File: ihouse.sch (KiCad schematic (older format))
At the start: 7 parts

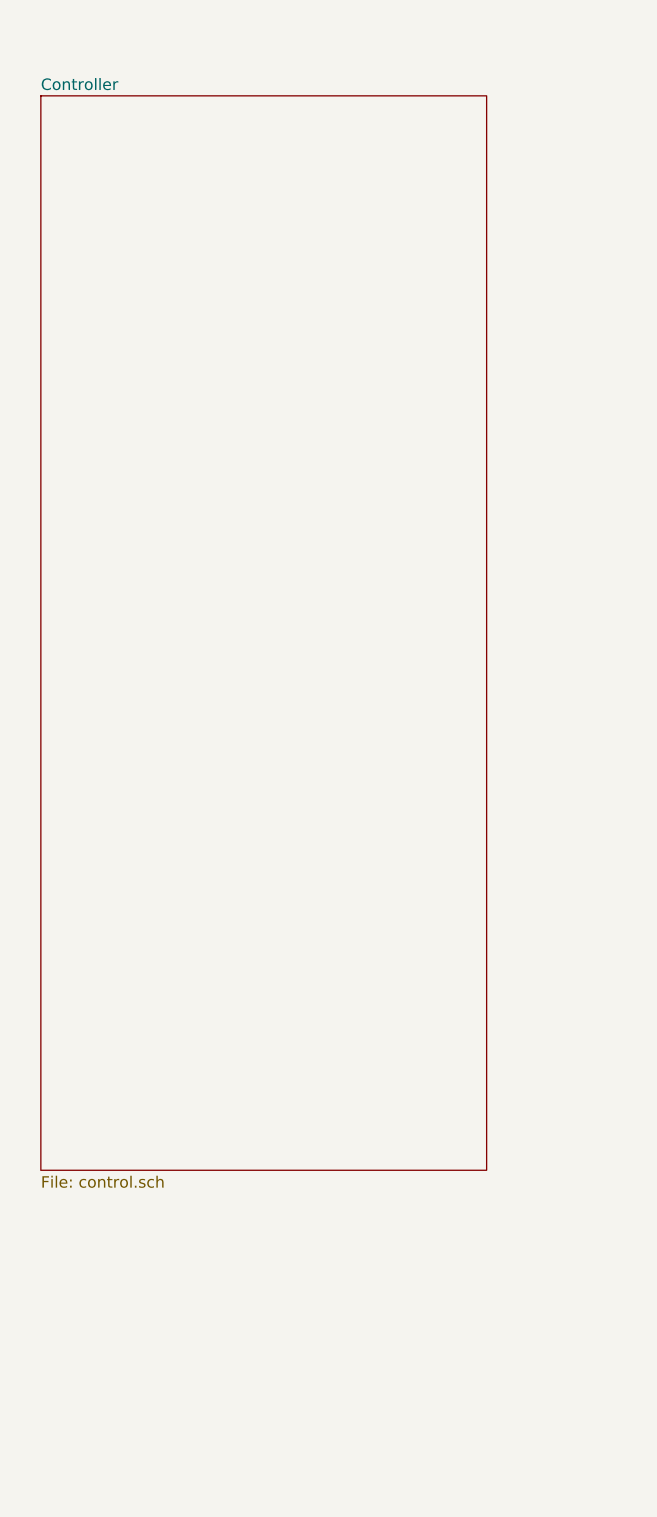
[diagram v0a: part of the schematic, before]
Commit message: tarpinis kommitas
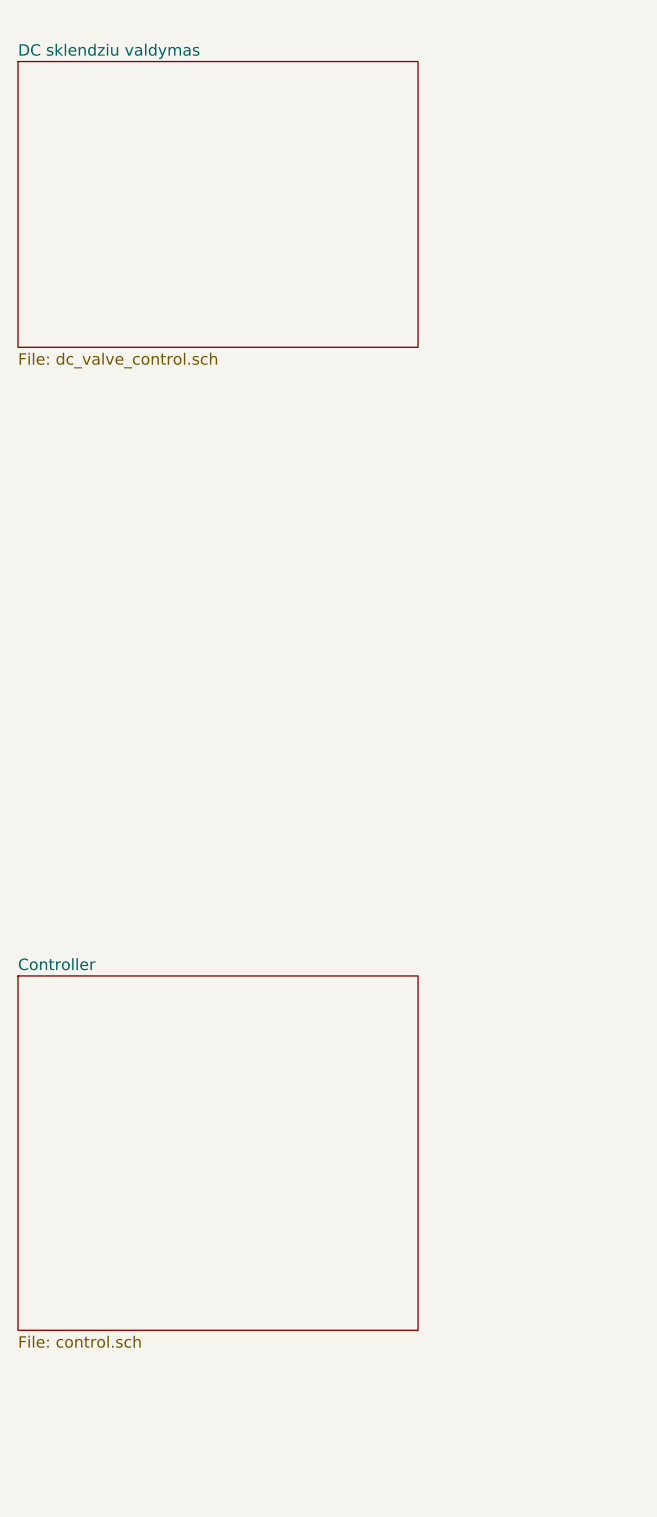
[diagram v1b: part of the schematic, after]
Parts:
- gave numbers to parts that had none: 7
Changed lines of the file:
@@
 $Descr A4 11693 8268
 encoding utf-8
-Sheet 1 3
+Sheet 1 4
 Title ""
 Date ""
@@
 $EndDescr
 $Sheet
-S 2100 1350 1950 4700
+S 2000 5200 1750 1550
 U 5BC6397F
 F0 "Controller" 50
@@
 PE
 $Comp
-L Connector_Generic:Conn_01x01 J?
+L Connector_Generic:Conn_01x01 J1
 U 1 1 5BC9AA2A
 P 10550 1600
-F 0 "J?" H 10630 1596 50  0000 L CNN
+F 0 "J1" H 10630 1596 50  0000 L CNN
 F 1 "Conn_01x01" H 10630 1551 50  0001 L CNN
 F 2 "mech:Faston_6.3x0.8x14" H 10550 1600 50  0001 C CNN
@@
 $EndComp
 $Comp
-L Connector_Generic:Conn_01x01 J?
+L Connector_Generic:Conn_01x01 J2
 U 1 1 5BC9AB40
 P 10550 1750
-F 0 "J?" H 10630 1746 50  0000 L CNN
+F 0 "J2" H 10630 1746 50  0000 L CNN
 F 1 "Conn_01x01" H 10630 1701 50  0001 L CNN
 F 2 "mech:Faston_6.3x0.8x14" H 10550 1750 50  0001 C CNN
@@
 $EndComp
 $Comp
-L Connector_Generic:Conn_01x01 J?
+L Connector_Generic:Conn_01x01 J3
 U 1 1 5BC9AB58
 P 10550 1900
-F 0 "J?" H 10630 1896 50  0000 L CNN
+F 0 "J3" H 10630 1896 50  0000 L CNN
 F 1 "Conn_01x01" H 10630 1851 50  0001 L CNN
 F 2 "mech:Faston_6.3x0.8x14" H 10550 1900 50  0001 C CNN
@@
 $EndComp
 $Comp
-L Connector_Generic:Conn_01x01 J?
+L Connector_Generic:Conn_01x01 J4
 U 1 1 5BC9AB72
 P 10550 2050
-F 0 "J?" H 10630 2046 50  0000 L CNN
+F 0 "J4" H 10630 2046 50  0000 L CNN
 F 1 "Conn_01x01" H 10630 2001 50  0001 L CNN
 F 2 "mech:Faston_6.3x0.8x14" H 10550 2050 50  0001 C CNN
@@
 	6400 4050 6700 4050
 $Comp
-L Connector_Generic:Conn_01x03 J?
+L Connector_Generic:Conn_01x03 J5
 U 1 1 5BC74B70
 P 10550 2550
-F 0 "J?" H 10630 2546 50  0000 L CNN
+F 0 "J5" H 10630 2546 50  0000 L CNN
 F 1 "Conn_01x03" H 10630 2501 50  0001 L CNN
 F 2 "Connectors_Phoenix:PhoenixContact_MSTBA-G_03x5.00mm_Angled" H 10550 2550 50  0001 C CNN
@@
 P 6050 5850
 AR Path="/5BC77CC5/5C039156" Ref="J?"  Part="1"
-AR Path="/5C039156" Ref="J?"  Part="1"
-F 0 "J?" H 6100 6450 50  0000 C CNN
+AR Path="/5C039156" Ref="J7"  Part="1"
+F 0 "J7" H 6100 6450 50  0000 C CNN
 F 1 "AC OUTS" H 6100 5150 50  0000 C CNN
 F 2 "Connector_Molex:Molex_Mini-Fit_Jr_5566-24A_2x12_P4.20mm_Vertical" H 6050 5850 50  0001 C CNN
@@
 P 7800 5350
 AR Path="/5BC77CC5/5C03917E" Ref="J?"  Part="1"
-AR Path="/5C03917E" Ref="J?"  Part="1"
-F 0 "J?" H 7850 5450 50  0000 C CNN
+AR Path="/5C03917E" Ref="J6"  Part="1"
+F 0 "J6" H 7850 5450 50  0000 C CNN
 F 1 "AC INPUTS" H 7850 5150 50  0000 C CNN
 F 2 "Connector_Molex:Molex_Mini-Fit_Jr_5566-04A_2x02_P4.20mm_Vertical" H 7800 5350 50  0001 C CNN
@@
 F36 "OAC9" I R 7900 2950 50
 $EndSheet
+$Sheet
+S 2000 1200 1750 1250
+U 5E405C96
+F0 "DC sklendziu valdymas" 50
+F1 "dc_valve_control.sch" 50
+$EndSheet
 $EndSCHEMATC

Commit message: tarpinis kommitas
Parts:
- J1: renamed from J7; symbol Connector_Generic:Conn_02x12_Counter_Clockwise -> ihouse-rescue:Connector_Generic_Conn_02x12_Counter_Clockwise-ihouse-rescue
- J2: renamed from J6; symbol Connector_Generic:Conn_02x02_Counter_Clockwise -> ihouse-rescue:Connector_Generic_Conn_02x02_Counter_Clockwise-ihouse-rescue
- J3: renamed from J1; symbol Connector_Generic:Conn_01x01 -> ihouse-rescue:Connector_Generic_Conn_01x01-ihouse-rescue
- J4: renamed from J2; symbol Connector_Generic:Conn_01x01 -> ihouse-rescue:Connector_Generic_Conn_01x01-ihouse-rescue
- J5: renamed from J3; symbol Connector_Generic:Conn_01x01 -> ihouse-rescue:Connector_Generic_Conn_01x01-ihouse-rescue
- J6: renamed from J4; symbol Connector_Generic:Conn_01x01 -> ihouse-rescue:Connector_Generic_Conn_01x01-ihouse-rescue
- J7: renamed from J5; symbol Connector_Generic:Conn_01x03 -> ihouse-rescue:Connector_Generic_Conn_01x03-ihouse-rescue
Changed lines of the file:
@@
 $EndSheet
 Wire Wire Line
-	6700 2150 6500 2150
-Wire Wire Line
-	6700 2250 6600 2250
+	6000 2150 6500 2150
+Wire Wire Line
+	6000 2250 6600 2250
 Text Label 6000 2150 0    50   ~ 0
 230VAC_L
@@
 Connection ~ 6500 2150
 Wire Wire Line
-	6500 2150 6000 2150
-Wire Wire Line
-	6600 2250 6600 1600
+	6600 1350 6600 1600
 Wire Wire Line
 	6600 1350 7300 1350
 Connection ~ 6600 2250
 Wire Wire Line
-	6600 2250 6000 2250
-Wire Wire Line
 	6500 1500 7300 1500
 Connection ~ 6500 1500
 Wire Wire Line
-	6500 1500 6500 1250
+	6500 1250 6500 1500
 Text Label 7300 1250 2    50   ~ 0
 OUTAC11
@@
 PE
 $Comp
-L Connector_Generic:Conn_01x01 J1
+L ihouse-rescue:Connector_Generic_Conn_01x01-ihouse-rescue J3
 U 1 1 5BC9AA2A
 P 10550 1600
-F 0 "J1" H 10630 1596 50  0000 L CNN
+F 0 "J3" H 10630 1596 50  0000 L CNN
 F 1 "Conn_01x01" H 10630 1551 50  0001 L CNN
 F 2 "mech:Faston_6.3x0.8x14" H 10550 1600 50  0001 C CNN
@@
 $EndComp
 $Comp
-L Connector_Generic:Conn_01x01 J2
+L ihouse-rescue:Connector_Generic_Conn_01x01-ihouse-rescue J4
 U 1 1 5BC9AB40
 P 10550 1750
-F 0 "J2" H 10630 1746 50  0000 L CNN
+F 0 "J4" H 10630 1746 50  0000 L CNN
 F 1 "Conn_01x01" H 10630 1701 50  0001 L CNN
 F 2 "mech:Faston_6.3x0.8x14" H 10550 1750 50  0001 C CNN
@@
 $EndComp
 $Comp
-L Connector_Generic:Conn_01x01 J3
+L ihouse-rescue:Connector_Generic_Conn_01x01-ihouse-rescue J5
 U 1 1 5BC9AB58
 P 10550 1900
-F 0 "J3" H 10630 1896 50  0000 L CNN
+F 0 "J5" H 10630 1896 50  0000 L CNN
 F 1 "Conn_01x01" H 10630 1851 50  0001 L CNN
 F 2 "mech:Faston_6.3x0.8x14" H 10550 1900 50  0001 C CNN
@@
 $EndComp
 $Comp
-L Connector_Generic:Conn_01x01 J4
+L ihouse-rescue:Connector_Generic_Conn_01x01-ihouse-rescue J6
 U 1 1 5BC9AB72
 P 10550 2050
-F 0 "J4" H 10630 2046 50  0000 L CNN
+F 0 "J6" H 10630 2046 50  0000 L CNN
 F 1 "Conn_01x01" H 10630 2001 50  0001 L CNN
 F 2 "mech:Faston_6.3x0.8x14" H 10550 2050 50  0001 C CNN
@@
 	10250 1600 10250 1750
 Wire Wire Line
-	10250 2050 10350 2050
-Wire Wire Line
-	10350 1900 10250 1900
+	9850 2050 10250 2050
+Wire Wire Line
+	10250 1900 10350 1900
 Connection ~ 10250 1900
 Wire Wire Line
-	10250 1900 10250 2050
-Wire Wire Line
-	10350 1750 10250 1750
+	10250 1750 10350 1750
 Connection ~ 10250 1750
-Wire Wire Line
-	10250 1750 10250 1900
-Wire Wire Line
-	10250 2050 9850 2050
 Connection ~ 10250 2050
 Text Label 9850 2050 0    50   ~ 0
@@
 	6400 4050 6700 4050
 $Comp
-L Connector_Generic:Conn_01x03 J5
+L ihouse-rescue:Connector_Generic_Conn_01x03-ihouse-rescue J7
 U 1 1 5BC74B70
 P 10550 2550
-F 0 "J5" H 10630 2546 50  0000 L CNN
+F 0 "J7" H 10630 2546 50  0000 L CNN
 F 1 "Conn_01x03" H 10630 2501 50  0001 L CNN
 F 2 "Connectors_Phoenix:PhoenixContact_MSTBA-G_03x5.00mm_Angled" H 10550 2550 50  0001 C CNN
@@
 OUTAC7
 $Comp
-L Connector_Generic:Conn_02x12_Counter_Clockwise J?
+L ihouse-rescue:Connector_Generic_Conn_02x12_Counter_Clockwise-ihouse-rescue J1
 U 1 1 5C039156
 P 6050 5850
-AR Path="/5BC77CC5/5C039156" Ref="J?"  Part="1"
-AR Path="/5C039156" Ref="J7"  Part="1"
-F 0 "J7" H 6100 6450 50  0000 C CNN
+F 0 "J1" H 6100 6450 50  0000 C CNN
 F 1 "AC OUTS" H 6100 5150 50  0000 C CNN
 F 2 "Connector_Molex:Molex_Mini-Fit_Jr_5566-24A_2x12_P4.20mm_Vertical" H 6050 5850 50  0001 C CNN
@@
 	6450 5750 6350 5750
 Wire Wire Line
-	6350 5650 6450 5650
+	6450 5650 6350 5650
 Connection ~ 6450 5650
 Wire Wire Line
-	6450 5650 6450 5750
-Wire Wire Line
-	6350 5550 6450 5550
+	6450 5550 6350 5550
 Connection ~ 6450 5550
 Wire Wire Line
-	6450 5550 6450 5650
-Wire Wire Line
-	6350 5450 6450 5450
+	6450 5450 6350 5450
 Connection ~ 6450 5450
-Wire Wire Line
-	6450 5450 6450 5550
-Wire Wire Line
-	6450 5350 6800 5350
 Connection ~ 6450 5350
 Wire Wire Line
@@
 	5850 5950 5450 5950
 Wire Wire Line
-	6350 5950 6450 5950
-Wire Wire Line
-	6450 5950 6450 5850
+	6450 5950 6350 5950
 Connection ~ 6450 5750
 Wire Wire Line
@@
 Connection ~ 6450 5850
 Wire Wire Line
-	6450 5850 6450 5750
-Wire Wire Line
 	7600 5350 7300 5350
 Wire Wire Line
@@
 	8100 5450 8400 5450
 $Comp
-L Connector_Generic:Conn_02x02_Counter_Clockwise J?
+L ihouse-rescue:Connector_Generic_Conn_02x02_Counter_Clockwise-ihouse-rescue J2
 U 1 1 5C03917E
 P 7800 5350
-AR Path="/5BC77CC5/5C03917E" Ref="J?"  Part="1"
-AR Path="/5C03917E" Ref="J6"  Part="1"
-F 0 "J6" H 7850 5450 50  0000 C CNN
+F 0 "J2" H 7850 5450 50  0000 C CNN
 F 1 "AC INPUTS" H 7850 5150 50  0000 C CNN
 F 2 "Connector_Molex:Molex_Mini-Fit_Jr_5566-04A_2x02_P4.20mm_Vertical" H 7800 5350 50  0001 C CNN
@@
 INACN2
 Wire Wire Line
-	6350 6050 6450 6050
-Wire Wire Line
-	6450 6050 6450 5950
+	6450 6050 6350 6050
 Connection ~ 6450 5950
 Wire Wire Line
@@
 OUTAC9
 Wire Wire Line
-	6350 6150 6450 6150
+	6450 6150 6350 6150
 Wire Wire Line
 	5850 6350 5450 6350
@@
 Text Label 6800 6250 2    50   ~ 0
 OUTAC10N
-Wire Wire Line
-	6450 6150 6450 6050
 Connection ~ 6450 6050
 Text Notes 7300 6000 0    50   ~ 0
@@
 INACN2
 Wire Wire Line
-	6500 1500 6500 2150
-Wire Wire Line
-	7300 1600 6600 1600
+	6600 1600 7300 1600
 Connection ~ 6600 1600
-Wire Wire Line
-	6600 1600 6600 1350
 $Sheet
 S 6700 2050 1200 2400
@@
 F1 "dc_valve_control.sch" 50
 $EndSheet
+Wire Wire Line
+	6500 2150 6700 2150
+Wire Wire Line
+	6600 2250 6700 2250
+Wire Wire Line
+	6500 1500 6500 2150
+Wire Wire Line
+	10250 1900 10250 2050
+Wire Wire Line
+	10250 1750 10250 1900
+Wire Wire Line
+	10250 2050 10350 2050
+Wire Wire Line
+	6450 5650 6450 5750
+Wire Wire Line
+	6450 5550 6450 5650
+Wire Wire Line
+	6450 5450 6450 5550
+Wire Wire Line
+	6450 5350 6800 5350
+Wire Wire Line
+	6450 5750 6450 5850
+Wire Wire Line
+	6450 5850 6450 5950
+Wire Wire Line
+	6450 5950 6450 6050
+Wire Wire Line
+	6450 6050 6450 6150
+Wire Wire Line
+	6600 1600 6600 2250
 $EndSCHEMATC
